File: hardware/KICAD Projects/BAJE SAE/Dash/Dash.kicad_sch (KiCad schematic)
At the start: 34 parts, among them J1 Conn_01x02, J10 14 Segment (3), J11 14 Segment (4), J2 CAN to outer connector, J3 Conn_01x06, J4 Servo 1 (RPM), J5 Servo 2 (Speed), J6 Button 1, J7 Button 2, J8 14 Segment (1), J9 14 Segment (2)

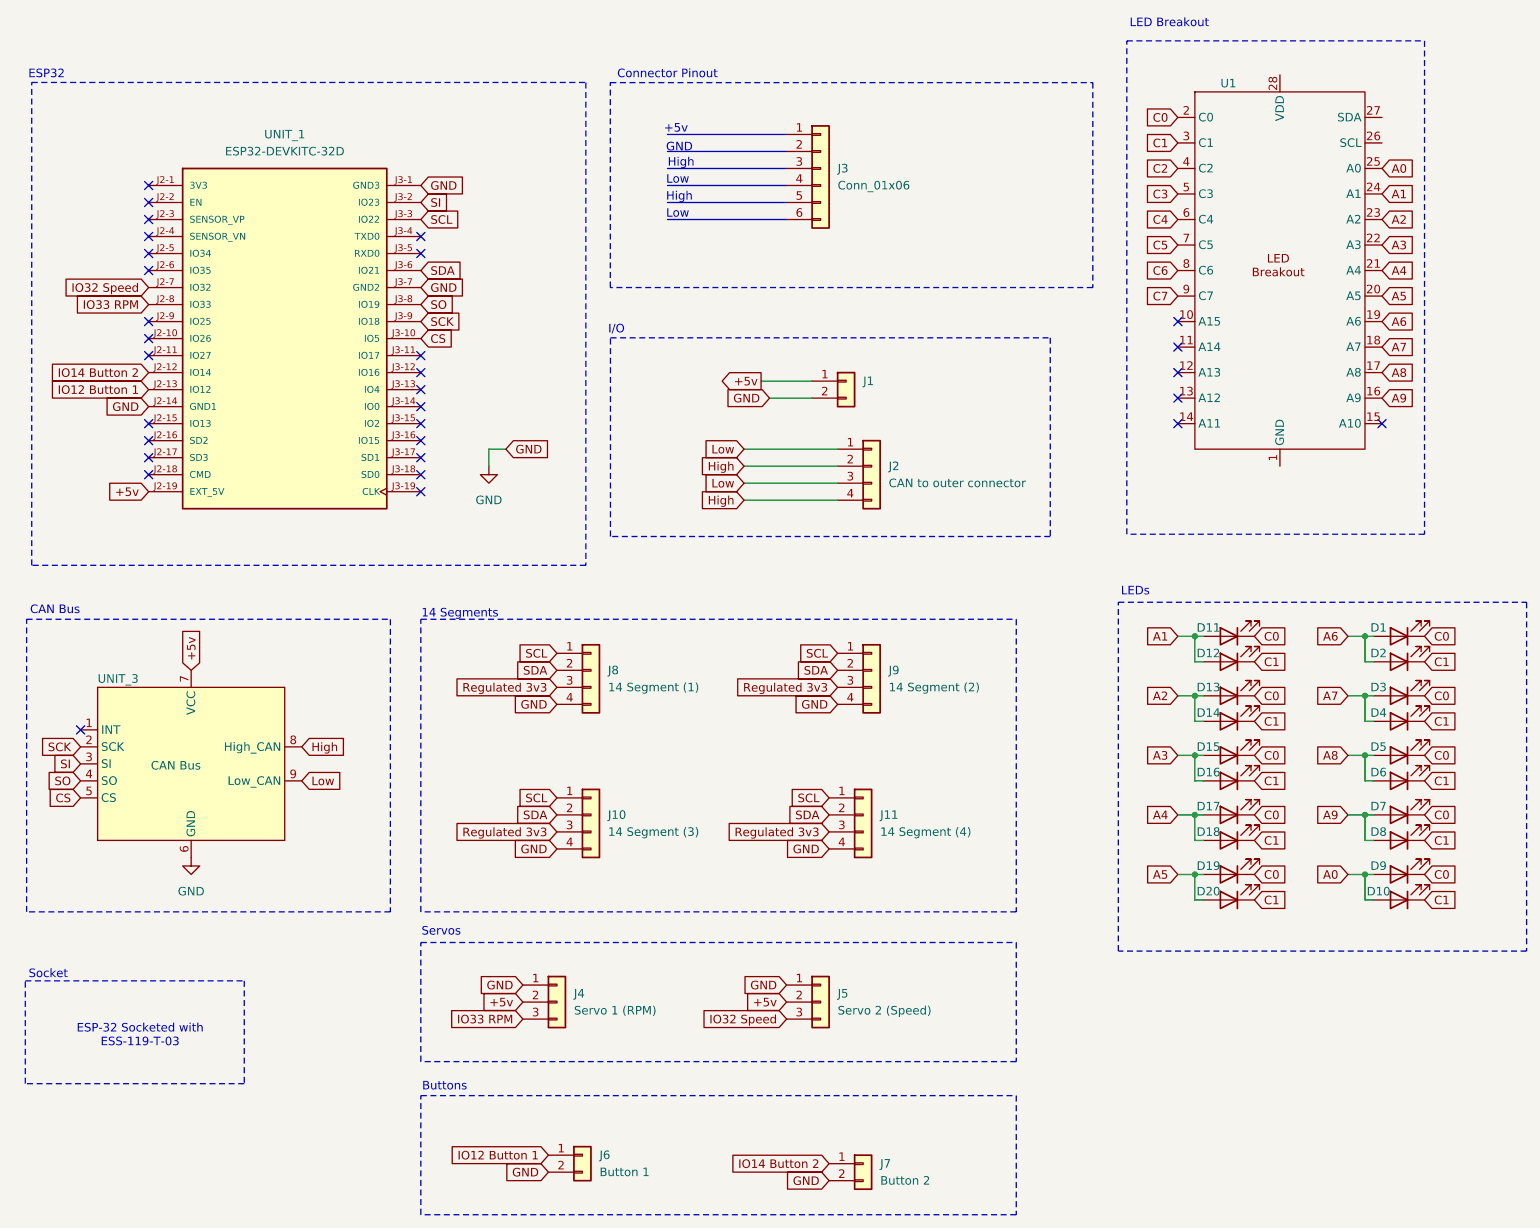
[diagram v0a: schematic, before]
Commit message: Added 3v3 voltage regulation
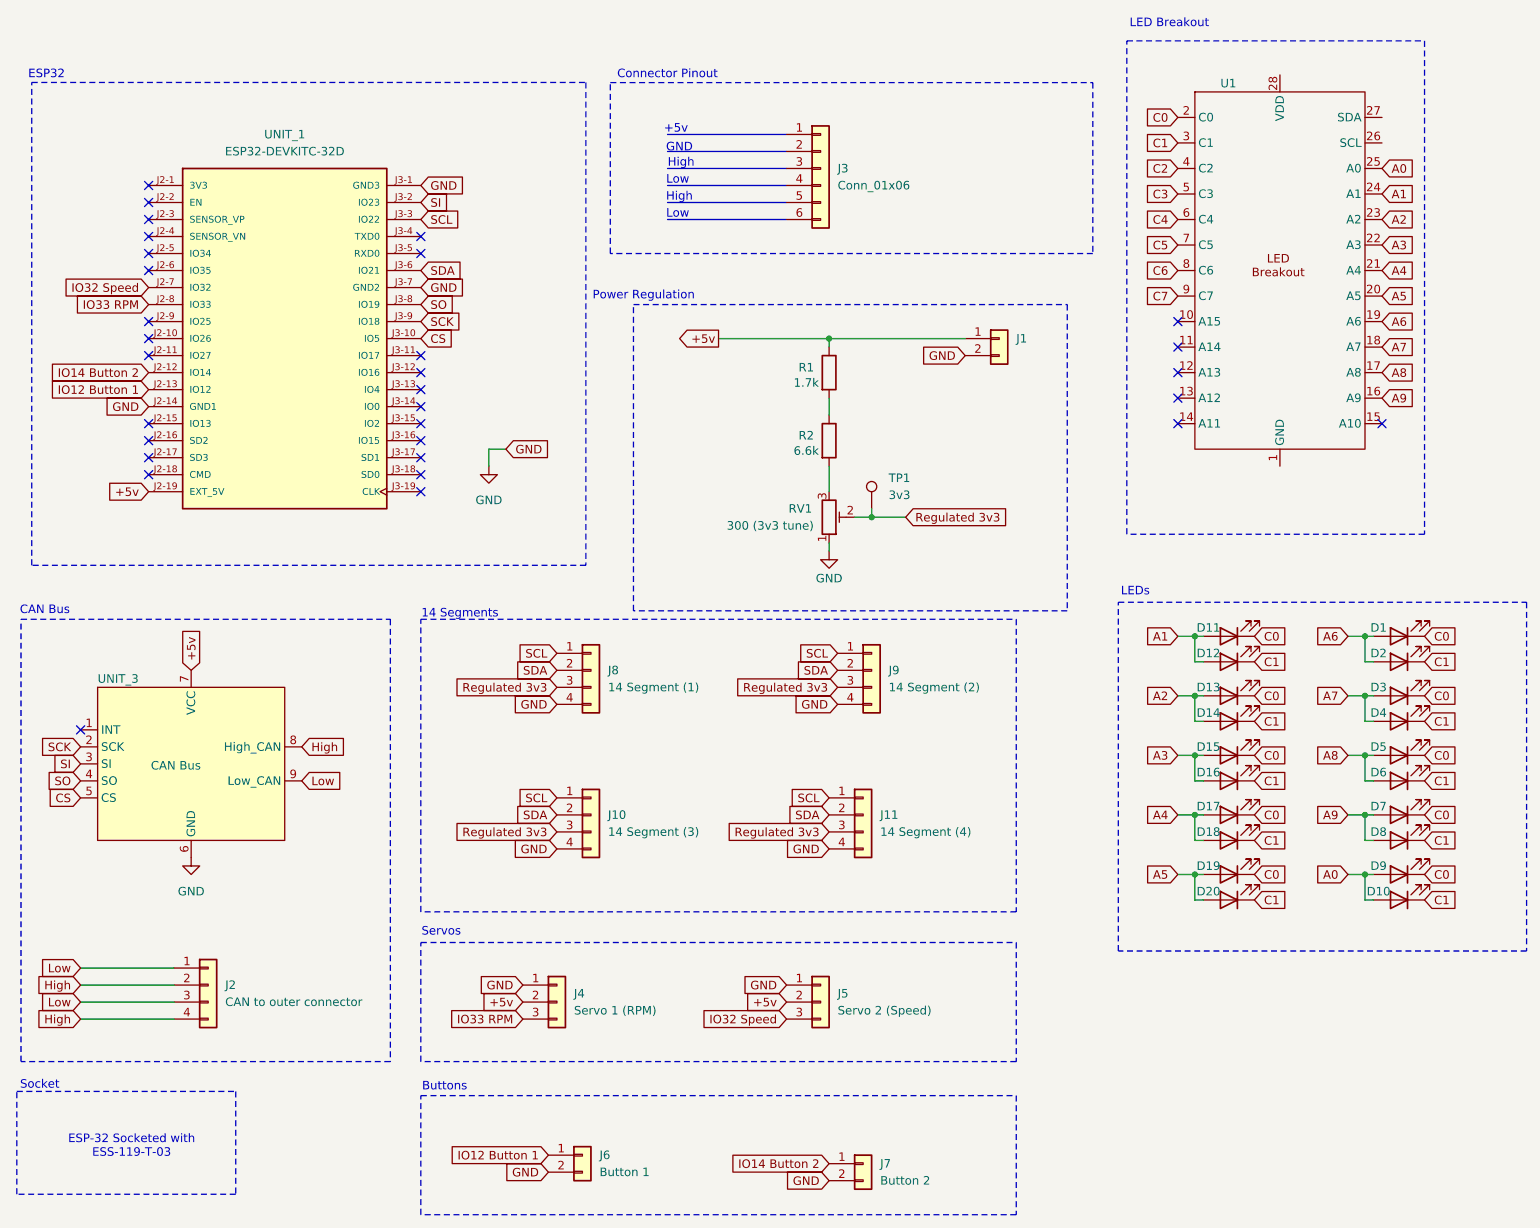
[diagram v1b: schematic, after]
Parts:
- added R1: 1.7k, symbol Device:R
- added R2: 6.6k, symbol Device:R
- added RV1: 300 (3v3 tune), symbol Device:R_Potentiometer_Trim
- added TP1: 3v3, symbol Connector:TestPoint
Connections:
- net +5v: now also R1.1
- net GND: now also RV1.1
- net Regulated 3v3: now also RV1.2, TP1.1
- new net: R2.2, RV1.3
- new net: R1.2, R2.1
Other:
- note added: "Power Regulation"
- note removed: "I/O"
- moved on the sheet: J1, J2
